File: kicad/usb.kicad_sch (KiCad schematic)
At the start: 5 parts, among them J8 USB_C_Receptacle_USB2.0_14P, U15 USBLC6-2SC6

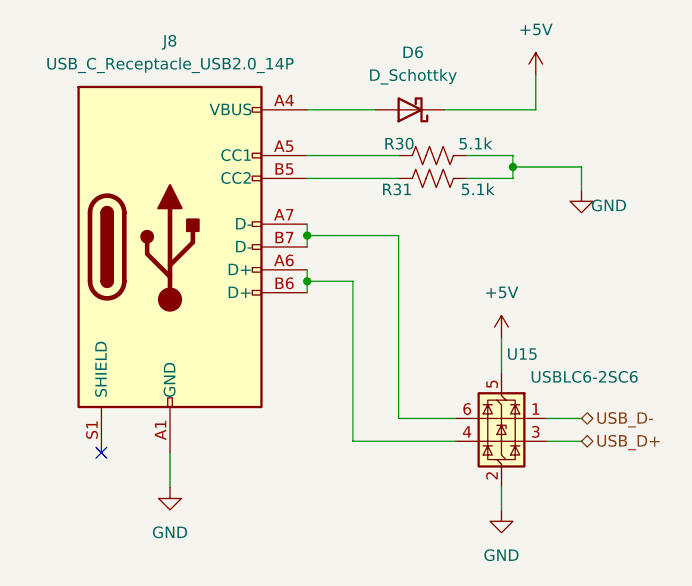
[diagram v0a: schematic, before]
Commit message: rev3 ordered
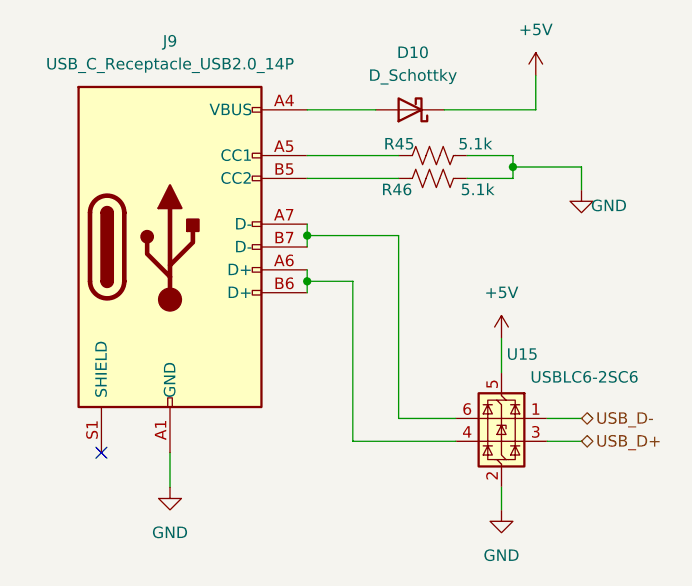
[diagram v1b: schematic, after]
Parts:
- renumbered D6 to D10, J8 to J9, R30 to R45, R31 to R46
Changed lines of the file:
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@@
 		(on_board yes)
 		(dnp no)
-		(property "Reference" "R30"
+		(property "Reference" "R45"
 			(at 119.888 76.2 90)
 			(effects
@@
 			(project "resc"
 				(path "/83aea3b7-5b9b-498e-8d41-e84fae2f87fa/5f81bd15-f3fb-48c3-8997-18d2496b9ffc"
-					(reference "R30")
+					(reference "R45")
 					(unit 1)
 				)
@@
 		(dnp no)
 		(fields_autoplaced yes)
-		(property "Reference" "#PWR076"
+		(property "Reference" "#PWR089"
 			(at 92.71 120.65 0)
 			(effects
@@
 			(project "resc"
 				(path "/83aea3b7-5b9b-498e-8d41-e84fae2f87fa/5f81bd15-f3fb-48c3-8997-18d2496b9ffc"
-					(reference "#PWR076")
+					(reference "#PWR089")
 					(unit 1)
 				)
@@
 		(dnp no)
 		(fields_autoplaced yes)
-		(property "Reference" "#PWR077"
+		(property "Reference" "#PWR090"
 			(at 129.54 123.19 0)
 			(effects
@@
 			(project "resc"
 				(path "/83aea3b7-5b9b-498e-8d41-e84fae2f87fa/5f81bd15-f3fb-48c3-8997-18d2496b9ffc"
-					(reference "#PWR077")
+					(reference "#PWR090")
 					(unit 1)
 				)
@@
 		(dnp no)
 		(fields_autoplaced yes)
-		(property "Reference" "#PWR075"
+		(property "Reference" "#PWR026"
 			(at 129.54 101.6 0)
 			(effects
@@
 			(project ""
 				(path "/83aea3b7-5b9b-498e-8d41-e84fae2f87fa/5f81bd15-f3fb-48c3-8997-18d2496b9ffc"
-					(reference "#PWR075")
+					(reference "#PWR026")
 					(unit 1)
 				)
@@
 		(dnp no)
 		(fields_autoplaced yes)
-		(property "Reference" "#PWR073"
+		(property "Reference" "#PWR086"
 			(at 133.35 72.39 0)
 			(effects
@@
 			(project ""
 				(path "/83aea3b7-5b9b-498e-8d41-e84fae2f87fa/5f81bd15-f3fb-48c3-8997-18d2496b9ffc"
-					(reference "#PWR073")
+					(reference "#PWR086")
 					(unit 1)
 				)
@@
 		(dnp no)
 		(fields_autoplaced yes)
-		(property "Reference" "D6"
+		(property "Reference" "D10"
 			(at 119.6975 66.04 0)
 			(effects
@@
 			(project ""
 				(path "/83aea3b7-5b9b-498e-8d41-e84fae2f87fa/5f81bd15-f3fb-48c3-8997-18d2496b9ffc"
-					(reference "D6")
+					(reference "D10")
 					(unit 1)
 				)
@@
 		(on_board yes)
 		(dnp no)
-		(property "Reference" "R31"
+		(property "Reference" "R46"
 			(at 119.634 81.28 90)
 			(effects
@@
 			(project "resc"
 				(path "/83aea3b7-5b9b-498e-8d41-e84fae2f87fa/5f81bd15-f3fb-48c3-8997-18d2496b9ffc"
-					(reference "R31")
+					(reference "R46")
 					(unit 1)
 				)
@@
 		(dnp no)
 		(fields_autoplaced yes)
-		(property "Reference" "J8"
+		(property "Reference" "J9"
 			(at 92.71 64.77 0)
 			(effects
@@
 			(project "resc"
 				(path "/83aea3b7-5b9b-498e-8d41-e84fae2f87fa/5f81bd15-f3fb-48c3-8997-18d2496b9ffc"
-					(reference "J8")
+					(reference "J9")
 					(unit 1)
 				)
@@
 		(on_board yes)
 		(dnp no)
-		(property "Reference" "#PWR074"
+		(property "Reference" "#PWR087"
 			(at 138.43 87.63 0)
 			(effects
@@
 			(project "resc"
 				(path "/83aea3b7-5b9b-498e-8d41-e84fae2f87fa/5f81bd15-f3fb-48c3-8997-18d2496b9ffc"
-					(reference "#PWR074")
-					(unit 1)
-				)
+					(reference "#PWR087")
+					(unit 1)
+				)
